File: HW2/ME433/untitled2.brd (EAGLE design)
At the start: 50 x 50 mm, 19 parts, among them SW1 DIP-SLIDE-SWITCH(3P-11.6X4.0X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

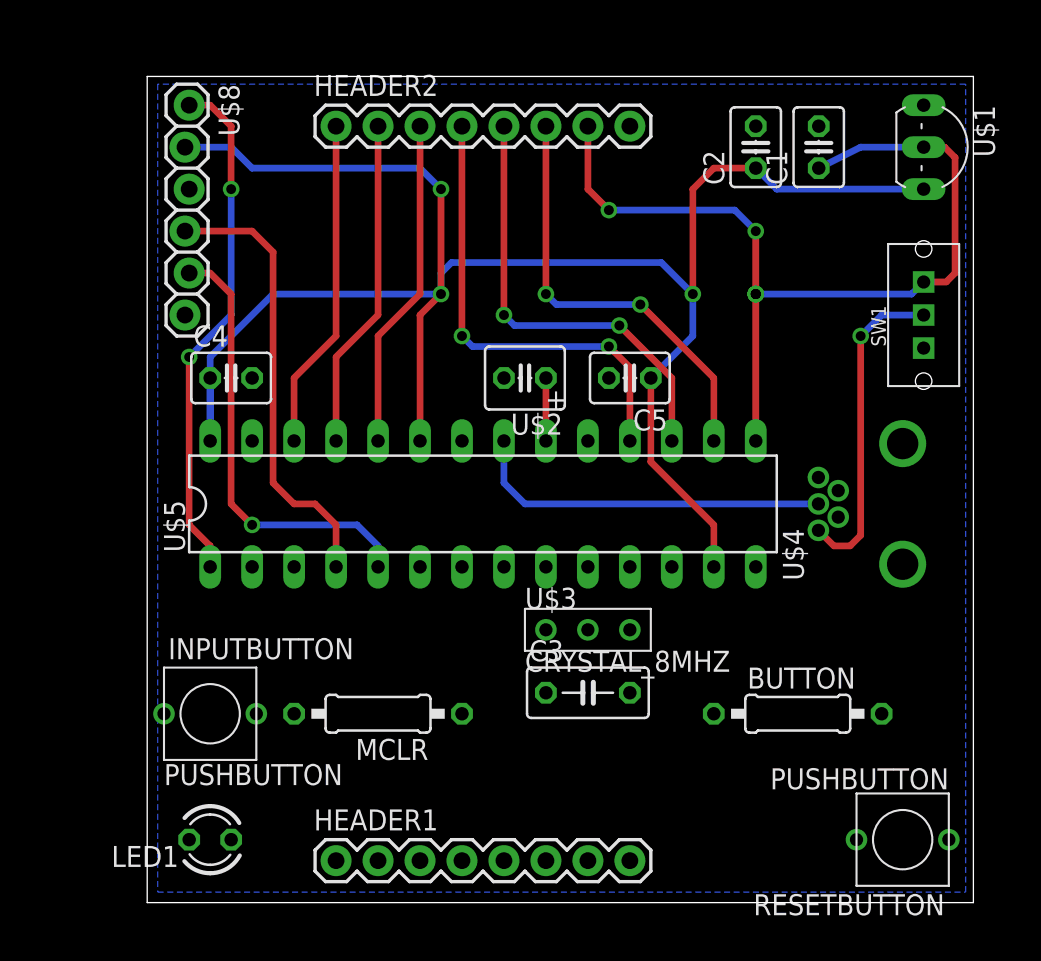
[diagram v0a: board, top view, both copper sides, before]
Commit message: presmash
layout complete, presmash and prenaming
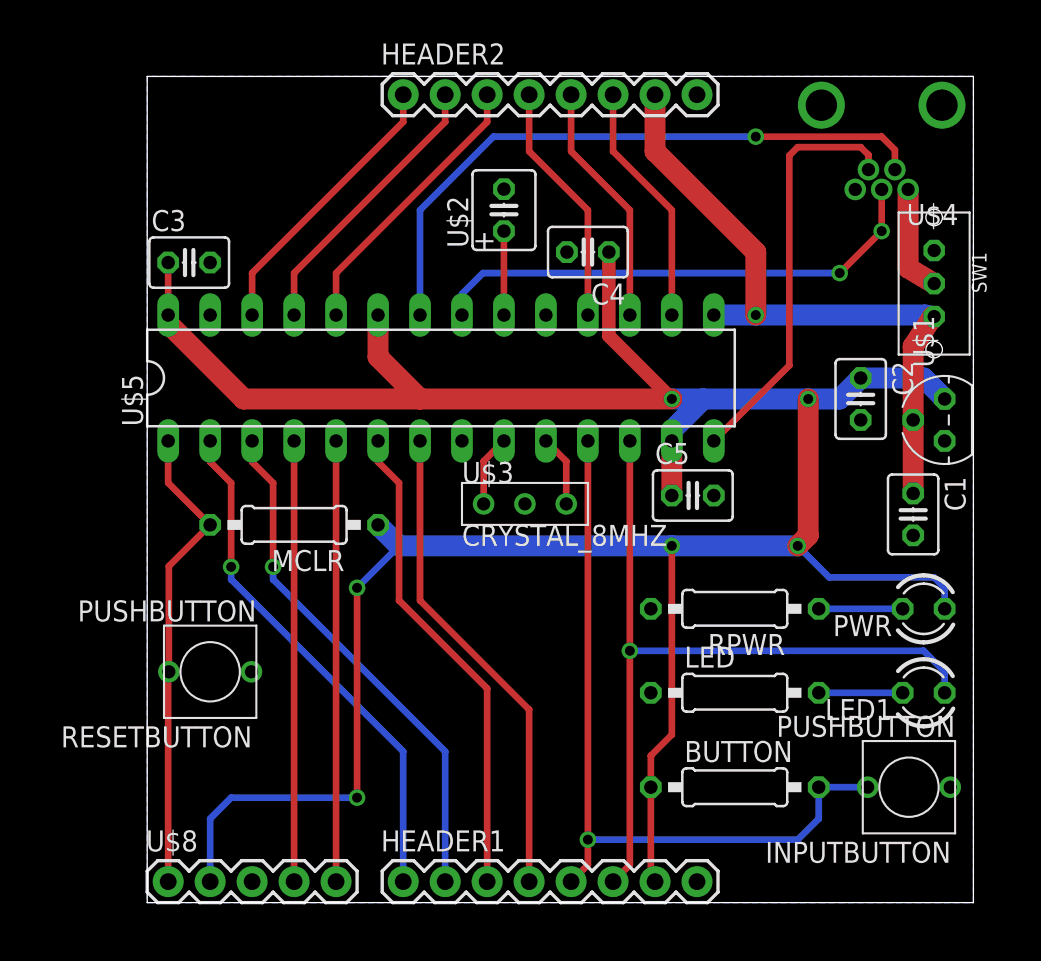
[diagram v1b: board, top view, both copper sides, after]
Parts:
- added LED, RPWR: 330, components:0207/10
- added PWR: RED, components:LED3MM
- C3: device components:C050-030X075 -> components:C025-030X050
- U$1: value VOLTAGE_REGULATOR_MCP1702 -> VOLTAGE_REGULATOR_MCP1702TO92; device components:TO92-EBC -> components:TO92
- U$8: value PICKITROW -> PICKITROW5ROW; device components:1X06_LOCK -> components:1X05
- moved U$8 47.0 mm to (1.27, 1.27), turned to 0 degrees
- moved LED1 44.1 mm to (47.0, 12.7)
- moved RESETBUTTON 43.1 mm to (3.81, 14.0)
- moved INPUTBUTTON 42.5 mm to (46.1, 6.99), turned to 180 degrees
- moved C3 35.5 mm to (2.54, 38.7)
- moved U$4 24.2 mm to (44.5, 48.3), turned to 270 degrees
- moved C1 22.9 mm to (46.4, 23.5), turned to 270 degrees
- moved C4 22.9 mm to (26.7, 39.4), turned to 180 degrees
- moved C2 16.5 mm to (43.2, 30.5), turned to 270 degrees
- moved U$1 16.5 mm to (48.3, 29.2), turned to 90 degrees
- moved MCLR 12.5 mm to (8.89, 22.9)
- moved U$2 10.2 mm to (21.6, 41.9), turned to 90 degrees
- moved U$3 8.52 mm to (22.9, 24.1)
- moved C5 8.07 mm to (33.0, 24.6), turned to 0 degrees
- moved U$5 8.03 mm to (17.8, 31.8)
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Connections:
- new net N$1: LED.2, LED1.K
- new net N$2: PWR.K, RPWR.1
- net +3V3: now also PWR.A, U$1.3; no longer U$1.E
- net +5V: now also U$1.2; no longer U$1.B
- net GND: now also LED.1, RPWR.2, U$1.1; no longer LED1.K, U$1.C
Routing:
- net +3V3: track 114.8 -> 173.6 mm, vias 3 -> 6
- net A4: track 0.00 -> 47.9 mm, vias 0 -> 1
- net B4: track 0.00 -> 46.5 mm, vias 0 -> 1
- net USBD-: track 0.00 -> 38.5 mm, vias 0 -> 1
- net A0: track 0.00 -> 31.5 mm, vias 0 -> 1
- net A1: track 0.00 -> 31.5 mm, vias 0 -> 1
- net B2: track 0.00 -> 29.4 mm
- net B3: track 0.00 -> 29.4 mm
- net USBID: track 0.00 -> 25.2 mm
- net +5V: track 56.1 -> 40.3 mm, vias 5 -> 1
- net B9: track 28.1 -> 14.8 mm, vias 2 -> 0
- net VBUS: track 19.6 -> 6.59 mm, vias 1 -> 0
- net B8: track 27.0 -> 14.8 mm, vias 2 -> 0
- net B7: track 26.2 -> 14.8 mm, vias 2 -> 0
- net USBD+: track 22.1 -> 30.8 mm, vias 0 -> 2
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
